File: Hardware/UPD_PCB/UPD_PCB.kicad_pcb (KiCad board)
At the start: 6 copper layers, 145 x 65 mm, 151 parts, among them IC1 STS30-DIS, J1 25A Fuse holder, J10 796739-2, J11 Conn_01x02, J12 Conn_01x01, J2 796739-2, J3 Conn_01x02, J4 1776119-2, J5 1776119-2, J6 1776119-2, J7 1776119-2, J8 1776119-2, J9 1776119-2, Q1 LMR51635XDDCR, Q2 LMR51635XDDCR, Q3 LMR51635XDDCR, Q4 LMR51635XDDCR, Q5 LMR51635XDDCR, Q6 LMR51635XDDCR, Q7 BSS84, U1 ACS711xEXLT-31AB, U2 INA219AxD, U3 INA219AxD, U4 INA219AxD, U5 INA219AxD, U6 INA219AxD, U7 INA219AxD

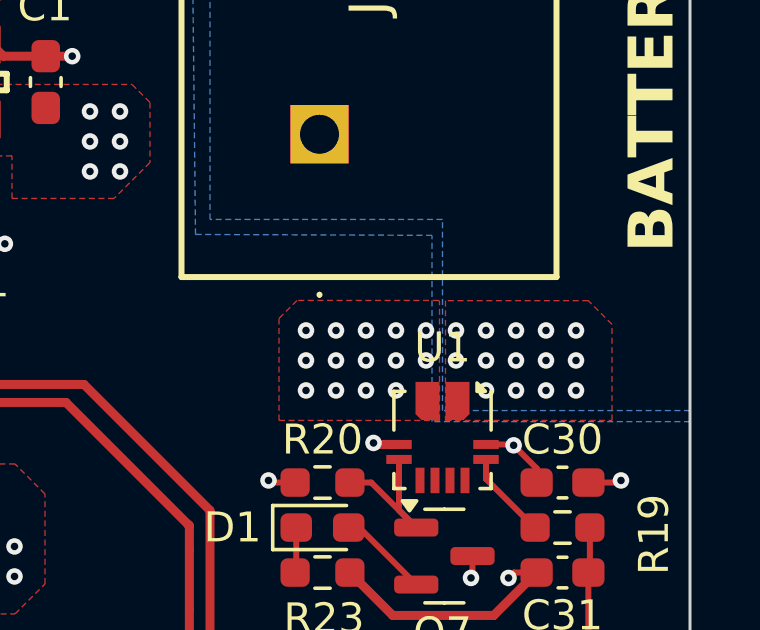
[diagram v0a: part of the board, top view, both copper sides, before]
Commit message: Updated pcb
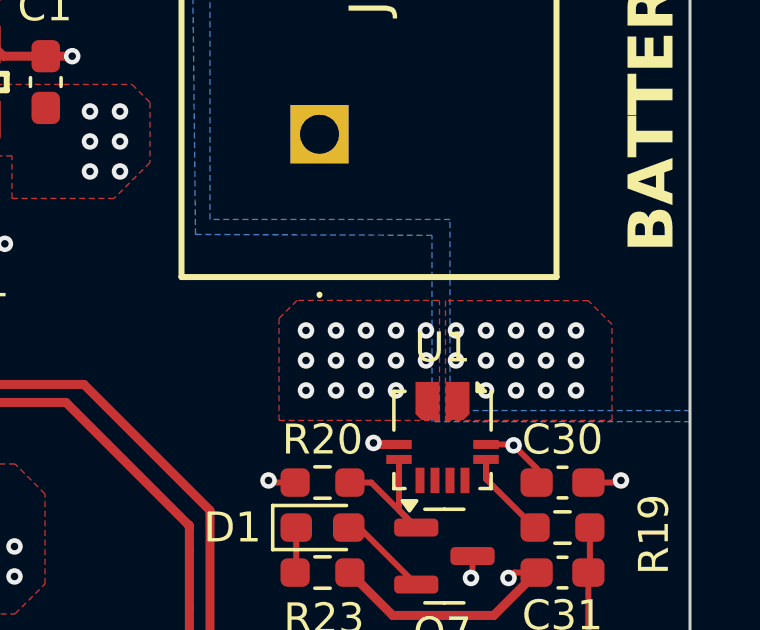
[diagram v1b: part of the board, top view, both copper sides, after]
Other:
- board text added: "0.0152mm"
- board text added: "0.035mm"
- board text added: "0.0994mm"
- board text added: "0.1088mm"
- board text added: "0.55mm"
- board text added: "L1 Sig"
- board text added: "L2 GND"
- board text added: "L3 Sig"
- board text added: "L4 PWR"
- board text added: "L5 GND"
- board text added: "L6 PWR"
- board text removed: "??? ??? ???"
- board text removed: "???mm"
- board text removed: "???mm (?oz)"
- board text removed: "ASSEMBLY NOTES (UNLESS OTHERWISE SPECIFIED) 1) DO NOT POPULATE PARTS ARE MARKED WITH A RED CROSS. 2) DO NOT POPULATE PARTS ARE NOT PRESENT IN THE BOM. 3) IF CONFLICTING INFORMATION IS FOUND BETWEEN THE ASSEMBLY FILE AND BOM, BOM SHOULD BE USED AS THE MAIN SOURCE."
- board text removed: "Back Side"
- board text removed: "Components"
- board text removed: "Front Side"
- board text removed: "L1 (Sig, PWR)"
- board text removed: "L2 (GND)"
- board text removed: "L3 (Sig, PWR)"
- board text removed: "L4 (Sig, PWR)"
- board text removed: "L5 (GND)"
- board text removed: "L6 (Sig, PWR)"
- board text removed: "THT SMD Total"
- board text removed: "Total"
